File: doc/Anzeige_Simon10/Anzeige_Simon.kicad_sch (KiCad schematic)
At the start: 25 parts, among them J1 I2C, J2 Daten, J3 MoGND, J4 Vcc, J5 AnzByte, U1 74HC688, U2 PCF8574P, U3 SFH617

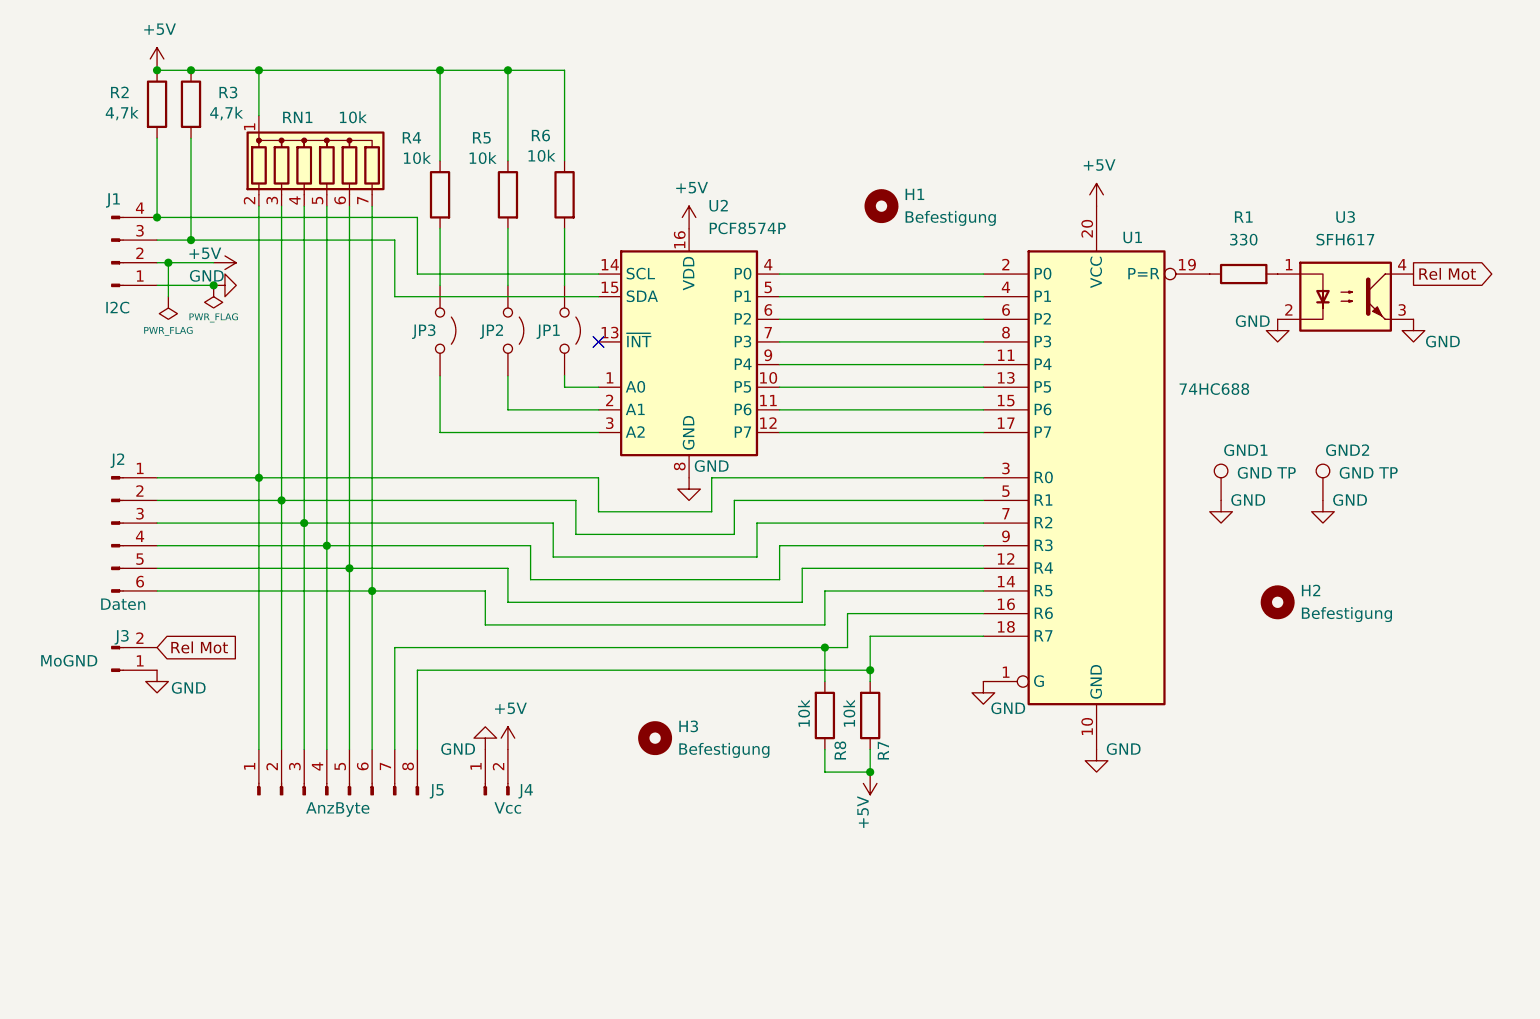
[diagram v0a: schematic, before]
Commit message: Update files
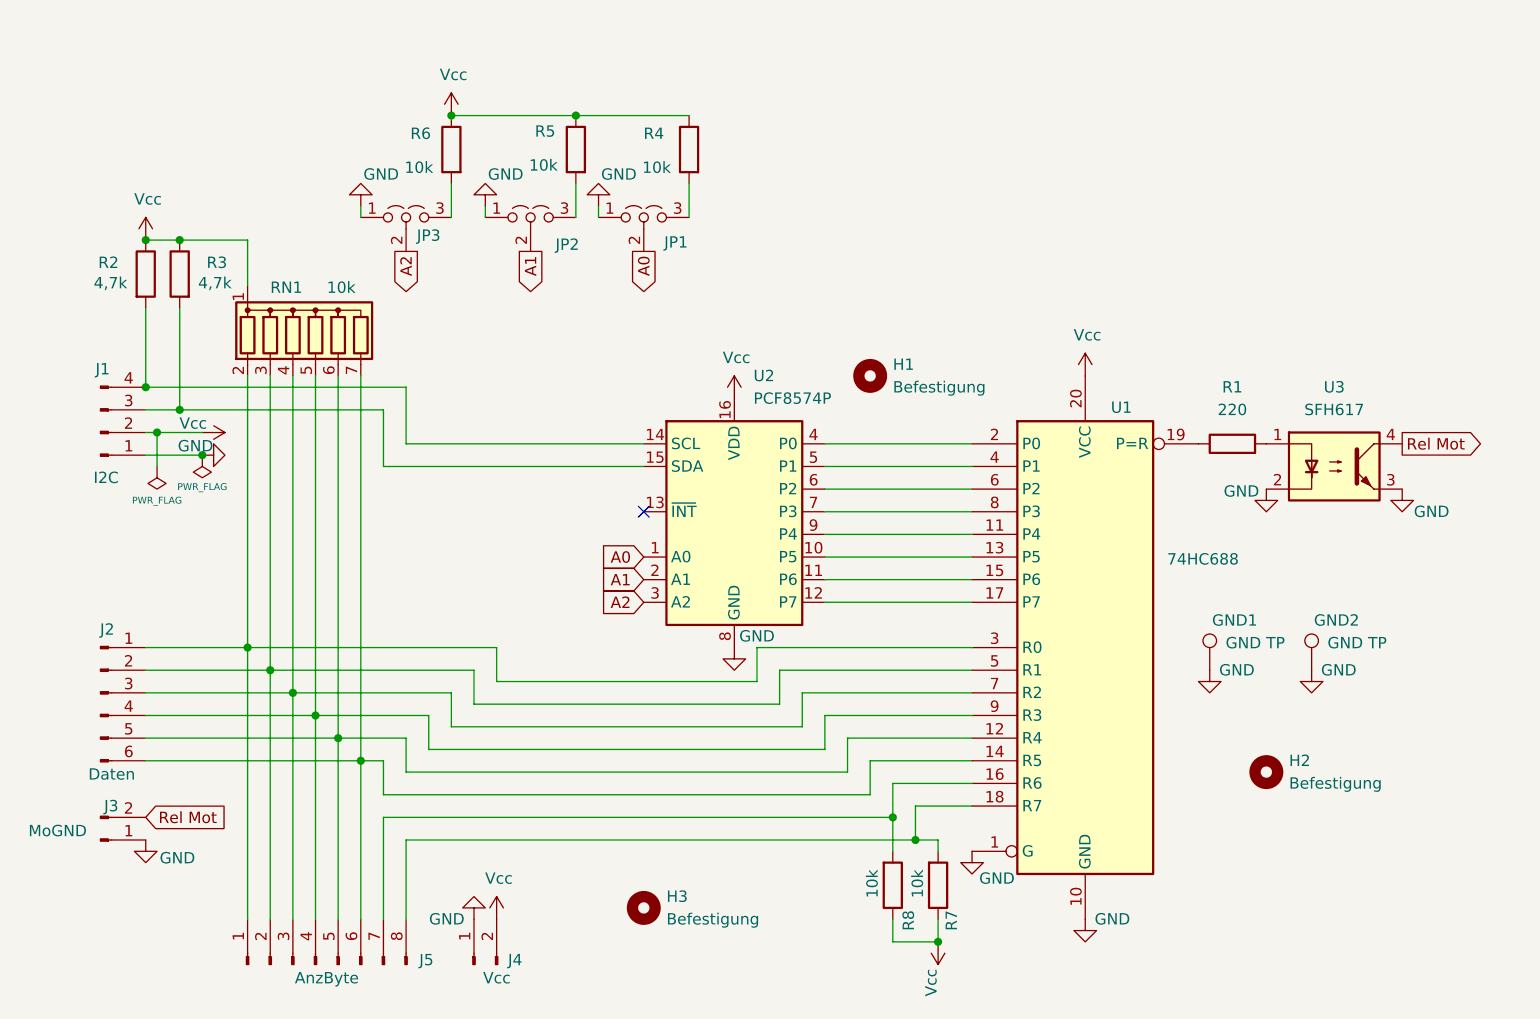
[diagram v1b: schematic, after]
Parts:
- removed JP1, JP2, JP3: (no value), Jumper:SolderJumper-2_P1.3mm_Open_RoundedPad1.0x1.5mm, symbol Jumper:Jumper_2_Open
- added JP1, JP2, JP3: Jumper_3_Open, Jumper:SolderJumper-3_P1.3mm_Open_RoundedPad1.0x1.5mm, symbol Jumper:Jumper_3_Open
- R1: value 330 -> 220
- renumbered R6 to R4, R4 to R6
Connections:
- net GND: now also JP1.1 (A), JP2.1 (A), JP3.1 (A)
- net at R5.2: now also JP2.3 (B)
- net A1: now reaches U2.2 (A1)
- net A1: now also JP2.2 (C)
- net at R4.2: now also JP1.3 (B)
- net A0: now reaches U2.1 (A0)
- net A0: now also JP1.2 (C)
- net A2: now reaches U2.3 (A2)
- net A2: now also JP3.2 (C)
- net at R6.2: now also JP3.3 (B)
- net +5V renamed Vcc
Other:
- moved on the sheet: GND1, GND2, H1, H2, H3, J1, J2, J3, J4, J5, R1, R2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

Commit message: Add files via upload
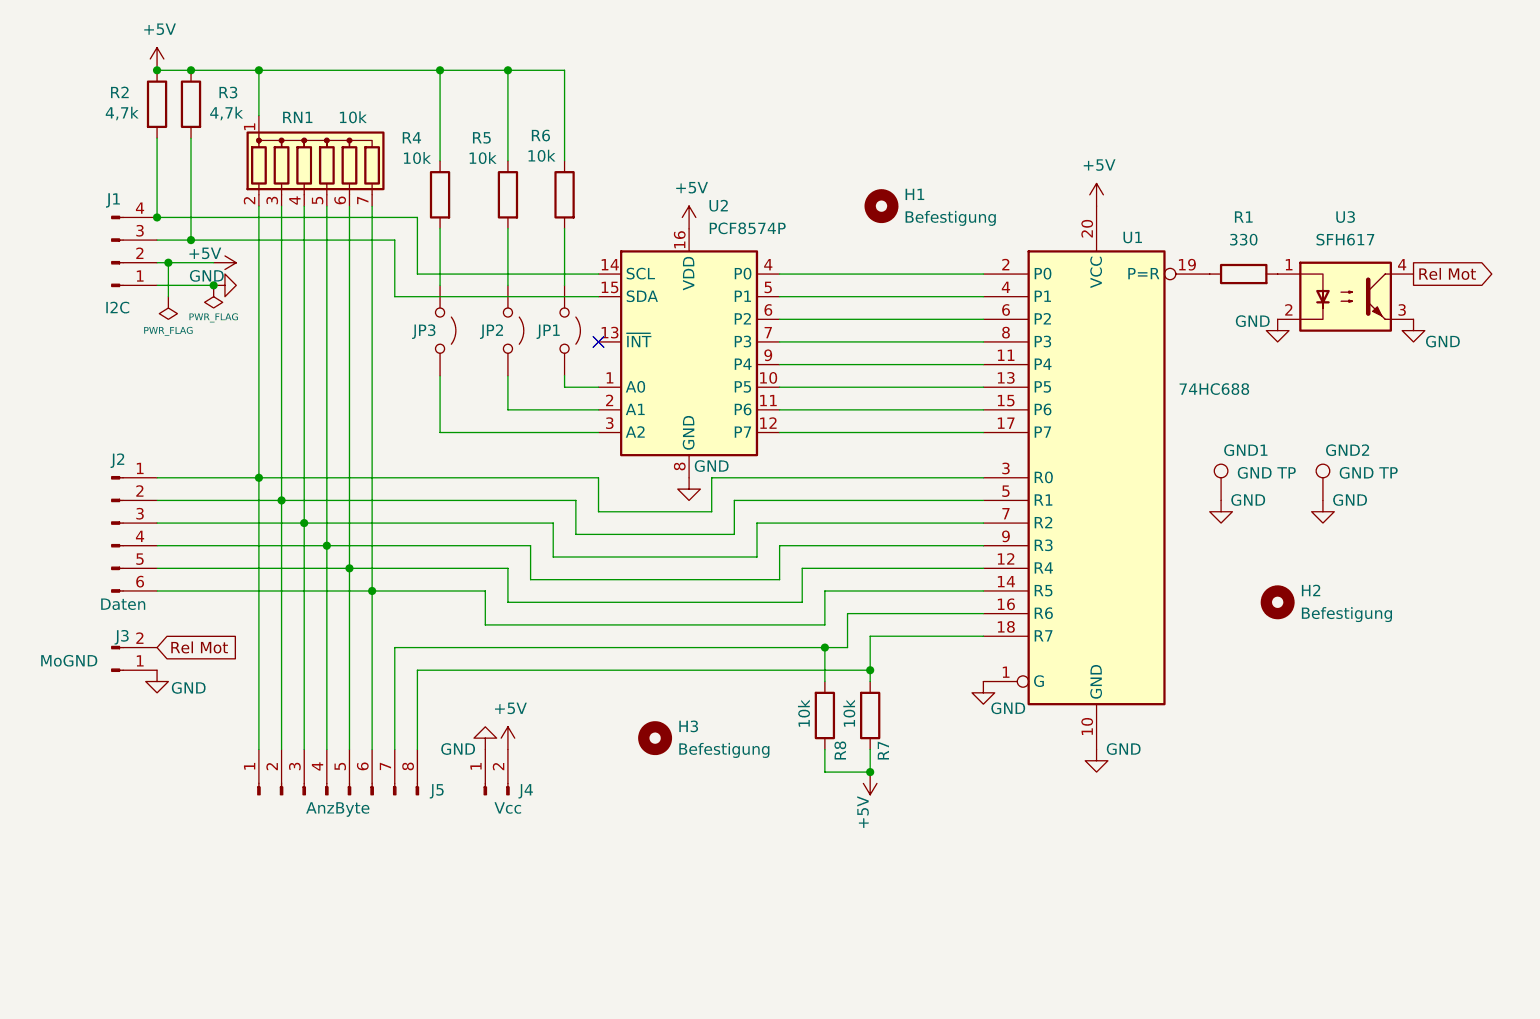
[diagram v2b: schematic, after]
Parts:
- removed JP1, JP2, JP3: Jumper_3_Open, Jumper:SolderJumper-3_P1.3mm_Open_RoundedPad1.0x1.5mm, symbol Jumper:Jumper_3_Open
- added JP1, JP2, JP3: (no value), Jumper:SolderJumper-2_P1.3mm_Open_RoundedPad1.0x1.5mm, symbol Jumper:Jumper_2_Open
- R1: value 220 -> 330
- renumbered R6 to R4, R4 to R6
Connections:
- net at R5.2: now also JP2.1 (A)
- net at R4.2: now also JP3.1 (A)
- net at R6.2: now also JP1.1 (A)
- net A0: no longer names the net of U2.1 (A0)
- net A0: now also JP1.2 (B)
- net A1: no longer names the net of U2.2 (A1)
- net A1: now also JP2.2 (B)
- net A2: no longer names the net of U2.3 (A2)
- net A2: now also JP3.2 (B)
- net Vcc renamed +5V
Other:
- moved on the sheet: GND1, GND2, H1, H2, H3, J1, J2, J3, J4, J5, R1, R2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
